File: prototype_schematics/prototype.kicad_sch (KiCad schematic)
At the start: 98 parts, among them J1 AudioJack3, J2 Conn_01x04, J3 Conn_Coaxial, U1 MAX2608EUT+T, U10 TA0411A, U2 SPX3819M5-L, U3 TLV61046ADB, U4 MAX2680AUT+, U5 CD74HC4046A, U6 BGA2802, U7 IS31AP4991A, U8 SPX3819M5-L-3-3, U9 PSA4-5043, Y1 ECS-96SMF21A30

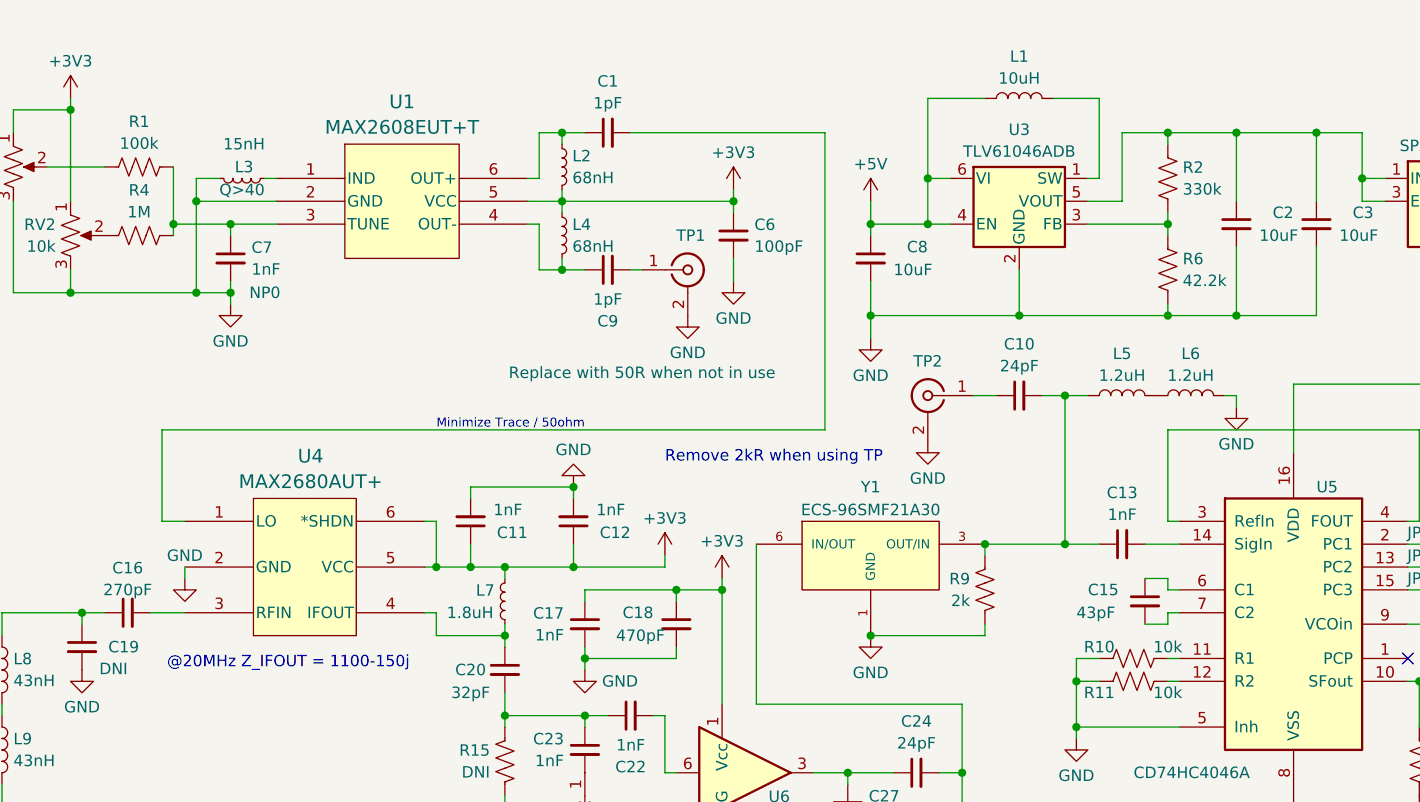
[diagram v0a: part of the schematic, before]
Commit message: layout wip
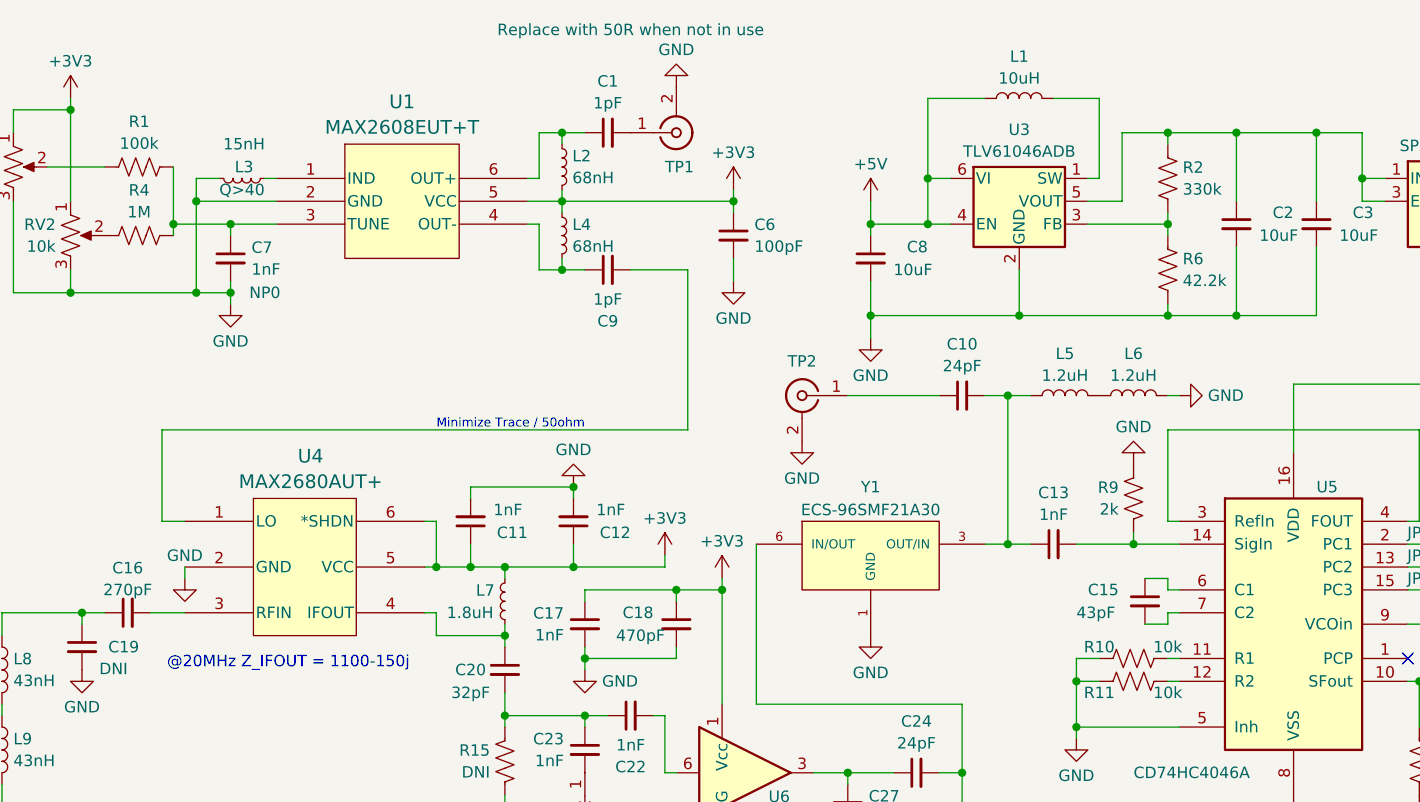
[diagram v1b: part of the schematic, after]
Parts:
- J3: footprint Connector_Coaxial:SMA_Wurth_60312002114503_Vertical -> Connector_Coaxial:SMA_Samtec_SMA-J-P-X-ST-EM1_EdgeMount; Digikey (none) -> CON-SMA-EDGE-S-ND
- L12: footprint Inductor_SMD:L_0201_0603Metric_Pad0.64x0.40mm_HandSolder -> Inductor_SMD:L_0603_1608Metric_Pad1.05x0.95mm_HandSolder
- TP1, TP2, TP3, TP4, TP5, TP6: footprint CONMHF1_SMD_T:CONN_CONMHF1-SMD_LNX -> Connector_Coaxial:U.FL_Molex_MCRF_73412-0110_Vertical
- U6: footprint Package_TO_SOT_SMD:SOT-363_SC-70-6 -> Package_TO_SOT_SMD:SOT-363_SC-70-6_Handsoldering
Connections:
- net GND: now also R9.1; no longer R9.2
- net at C10.2, C13.1, L5.1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: no longer R9.1
- net at C9.2: now also U4.1 (LO); no longer TP1.1 (In)
- net at C1.2: now also TP1.1 (In); no longer U4.1 (LO)
- net at C13.2, U5.14 (SigIn): now also R9.2
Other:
- note removed: "Remove 2kR when using TP"
- moved on the sheet: C10, C13, L5, L6, R9, TP1, TP2
